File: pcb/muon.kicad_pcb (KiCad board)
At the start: 2 copper layers, 54 x 39 mm, 18 parts, among them J1 Debug Pins, J2 USB_C_Receptacle_USB2.0, SW1 SW_SPST, SW2 SW_SPST, U1 ATSAMD11C14A-SS, U2 MIC5528-3.3YMT-TR

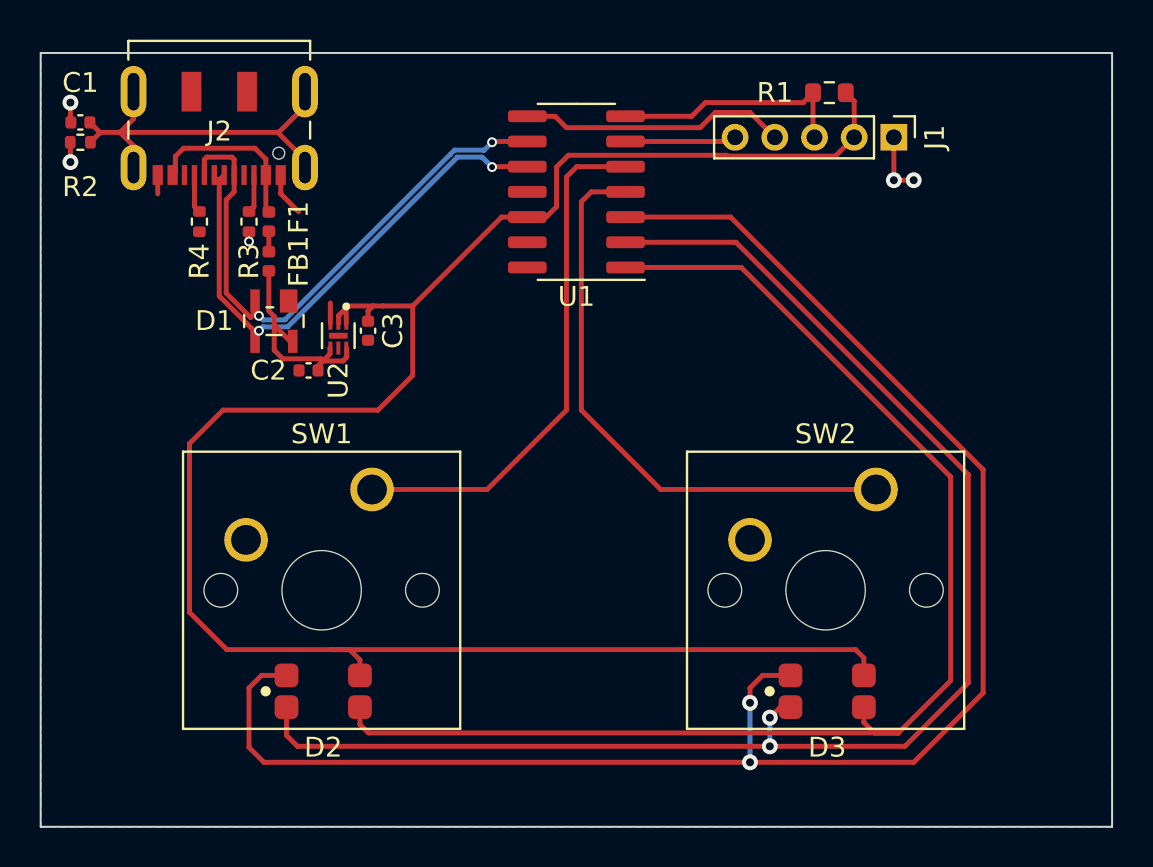
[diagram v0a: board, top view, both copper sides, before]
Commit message: re-route again
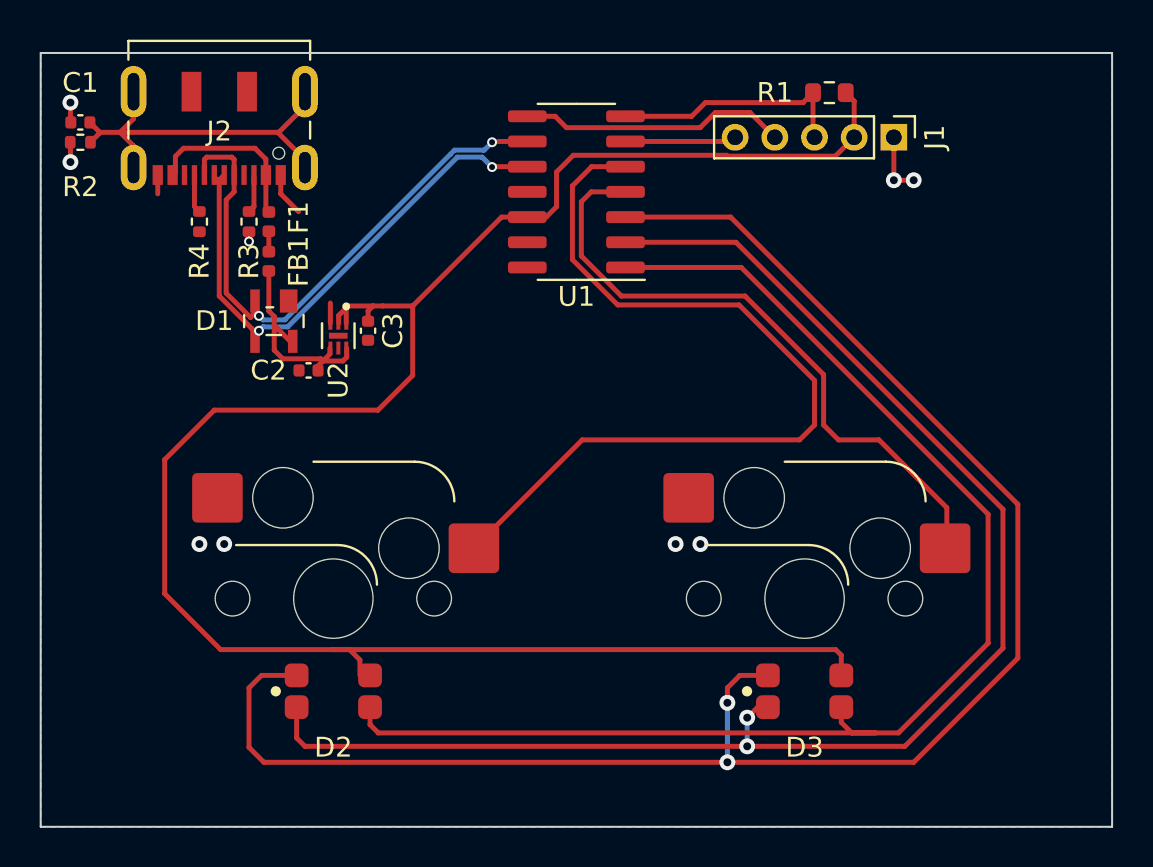
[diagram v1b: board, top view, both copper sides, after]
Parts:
- SW1, SW2: footprint Button_Switch_Keyboard:SW_Cherry_MX_1.25u_PCB -> Keyswitch:SW_Hotswap_Kailh_MX_1.25u; moved to B.Cu
- moved SW2 6.57 mm to (166.5, 85.5), turned to 180 degrees
- moved SW1 5.84 mm to (142.8, 85.5), turned to 180 degrees
- moved D3 1.14 mm to (166.5, 90.2)
- moved D2 0.51 mm to (142.8, 90.2)
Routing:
- net /SW1: track 26.4 -> 43.5 mm
- net /SW2: track 29.4 -> 32.4 mm
- net /LED_R: track 84.5 -> 86.5 mm
- net /LED_B: track 65.7 -> 66.7 mm
- net /LED_G: track 72.7 -> 73.7 mm
- net GND: vias 5 -> 9
